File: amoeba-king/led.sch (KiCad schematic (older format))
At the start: 1 part

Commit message: Getting closer
3d View still has pins :(
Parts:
- removed LED1: SK6812MINI, amoeba-modules:LED_SK6812MINI_E_PLCC4_3.2x2.8mm_Shine_Through, symbol LED:SK6812MINI
- added LED: SK6812MINI_E, amoeba-modules:LED_SK6812MINI_E_PLCC4_3.2x2.8mm_Shine_Through, symbol amoeba-royale-rescue:SK6812MINI_E
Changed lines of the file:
@@
 Text HLabel 6000 3650 2    60   Output ~ 0
 DOUT0
-$Comp
-L LED:SK6812MINI LED1
-U 1 1 5CC2CD58
-P 5600 3650
-F 0 "LED1" H 5850 3450 50  0000 L CNN
-F 1 "SK6812MINI" H 5850 3350 50  0000 L CNN
-F 2 "amoeba-modules:LED_SK6812MINI_E_PLCC4_3.2x2.8mm_Shine_Through" H 5650 3350 50  0001 L TNN
-F 3 "https://cdn-shop.adafruit.com/product-files/2686/SK6812MINI_REV.01-1-2.pdf" H 5700 3275 50  0001 L TNN
-	1    5600 3650
-	1    0    0    -1
-$EndComp
 Wire Wire Line
 	5600 3250 5600 3350
@@
 Wire Wire Line
 	5600 3950 5600 4050
+$Comp
+L amoeba-royale-rescue:SK6812MINI_E LED
+U 1 1 5EC279EC
+P 5600 3650
+F 0 "LED" H 5944 3696 50  0000 L CNN
+F 1 "SK6812MINI_E" H 5944 3605 50  0000 L CNN
+F 2 "amoeba-modules:LED_SK6812MINI_E_PLCC4_3.2x2.8mm_Shine_Through" H 5650 3350 50  0001 L TNN
+F 3 "https://cdn-shop.adafruit.com/product-files/2686/SK6812MINI_REV.01-1-2.pdf" H 5700 3275 50  0001 L TNN
+	1    5600 3650
+	1    0    0    -1
+$EndComp
 $EndSCHEMATC

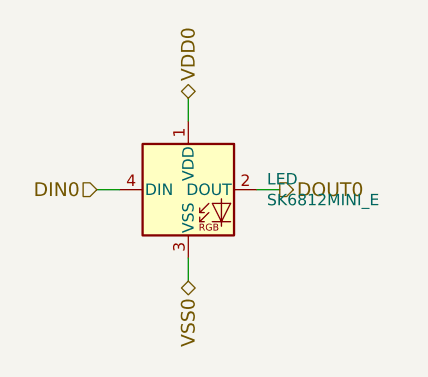
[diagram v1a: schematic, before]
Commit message: Getting ready for final review, before sending for production
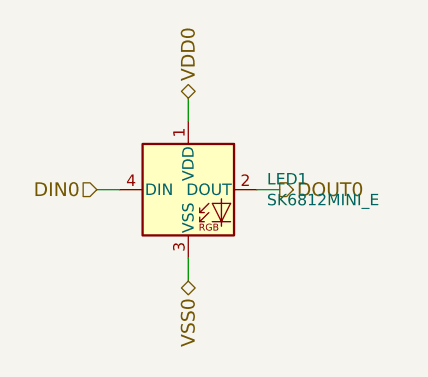
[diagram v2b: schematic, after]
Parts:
- renumbered LED to LED1
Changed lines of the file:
@@
 	5600 3950 5600 4050
 $Comp
-L amoeba-royale-rescue:SK6812MINI_E LED
+L amoeba-royale-rescue:SK6812MINI_E LED1
 U 1 1 5EC279EC
 P 5600 3650
-F 0 "LED" H 5944 3696 50  0000 L CNN
+F 0 "LED1" H 5944 3696 50  0000 L CNN
 F 1 "SK6812MINI_E" H 5944 3605 50  0000 L CNN
 F 2 "amoeba-modules:LED_SK6812MINI_E_PLCC4_3.2x2.8mm_Shine_Through" H 5650 3350 50  0001 L TNN

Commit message: Various Layout Improvements
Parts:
- LED1: symbol amoeba-royale-rescue:SK6812MINI_E -> amoeba-king-rescue:SK6812MINI_E-amoeba-royale-rescue
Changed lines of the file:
@@
 	5600 3950 5600 4050
 $Comp
-L amoeba-royale-rescue:SK6812MINI_E LED1
+L amoeba-king-rescue:SK6812MINI_E-amoeba-royale-rescue LED1
 U 1 1 5EC279EC
 P 5600 3650
